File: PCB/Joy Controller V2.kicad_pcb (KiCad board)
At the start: 2 copper layers, 172.6 x 70.1 mm, 78 parts, among them J1 USB_C_Receptacle_USB2.0_16P, J2 Conn_02x16_Odd_Even, Q1 NPN, Q2 NPN, SW1 SW_Push, SW10 SW_Push, SW11 SW_Push, SW12 SW_Push, SW13 SW_Push, SW14 RotaryEncoder_Switch_MP, SW2 SW_Push, SW3 SW_Push, SW4 SW_Push, SW5 SW_Push, SW6 SW_Push, SW7 SW_Push, SW8 SW_Push, SW9 SW_Push, U1 COM-09032, U2 COM-09032, U3 MCP23017_SO, U4 ADS1015IDGS

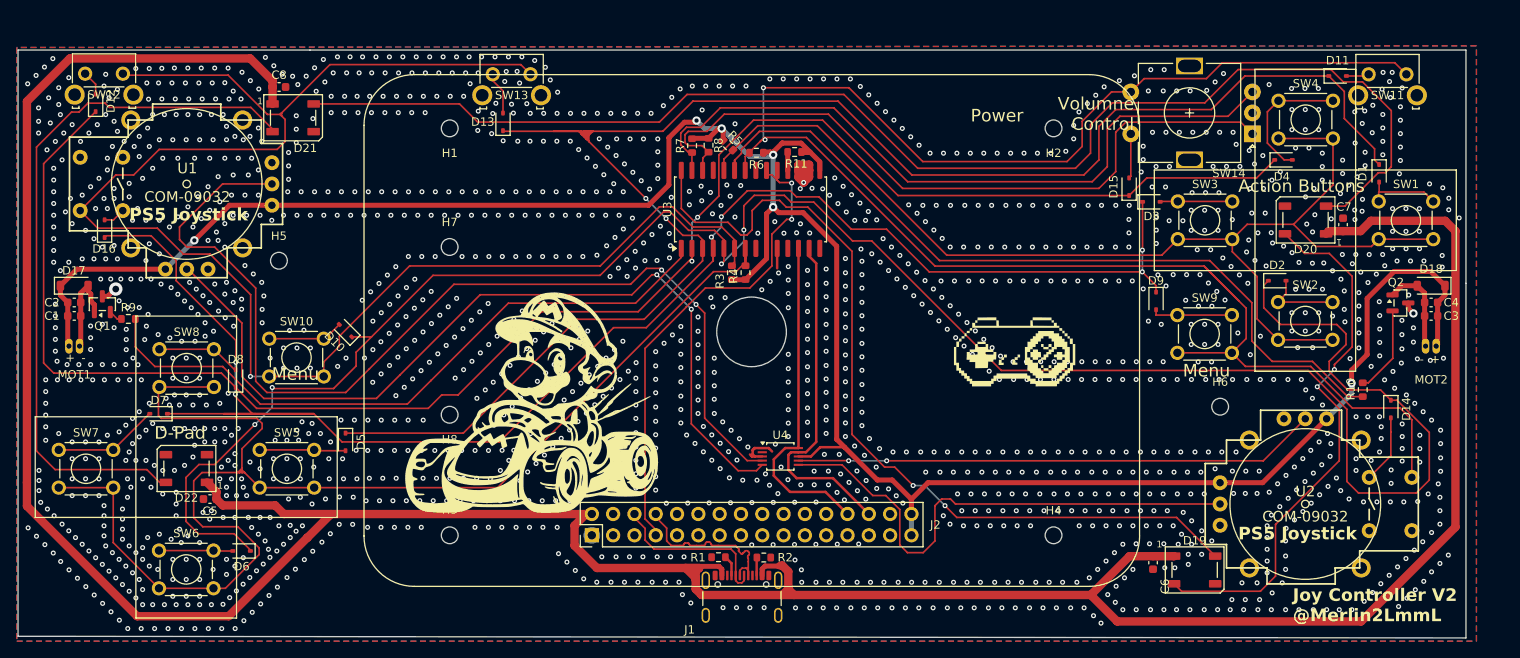
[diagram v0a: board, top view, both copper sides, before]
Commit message: Add files via upload
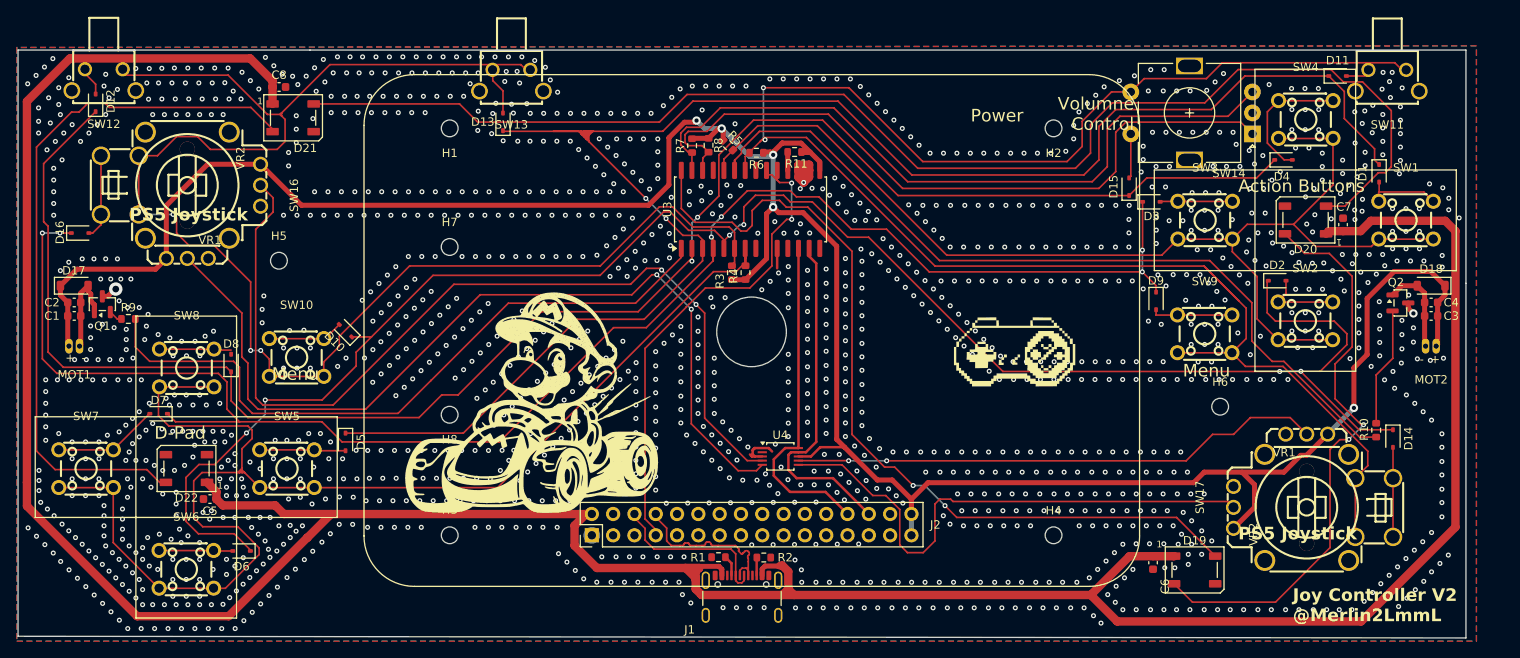
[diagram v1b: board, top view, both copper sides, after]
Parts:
- removed U1, U2: COM-09032, Joy:JOYSTICK
- added SW16: RKJXV1224005, lcsc:SW-TH_RKJXV1224005, F.Cu at (75.5, 81.0)
- added SW17: RKJXV1224005, lcsc:SW-TH_RKJXV1224005, F.Cu at (210.5, 117.0)
- SW1, SW10, SW2, SW3, SW4, SW5, SW6, SW7, SW8, SW9: value SW_Push -> B3F-1070; footprint Button_Switch_THT:SW_TH_Tactile_Omron_B3F-107x -> lcsc:SW-TH_4P-L6.2-W6.2-P4.50-LS6.5
- SW11, SW12, SW13: value SW_Push -> B3F-3152; footprint Button_Switch_THT:SW_SPST_Omron_B3F-315x_Angled -> lcsc:KEY-TH_4P-L7.3-W10.2-P4.50-LS7.0
- moved R10 5.08 mm to (218.0, 109.0)
- moved SW10 3.95 mm to (89.3, 100.3)
- moved SW3 3.95 mm to (197.6, 84.0)
- moved SW4 3.95 mm to (209.6, 72.0)
- moved SW5 3.95 mm to (88.2, 113.6)
- moved SW6 3.95 mm to (76.2, 125.6)
- moved SW7 3.95 mm to (64.2, 113.6)
- moved SW8 3.95 mm to (76.2, 101.6)
- moved SW1 3.95 mm to (221.6, 84.0)
- moved SW2 3.95 mm to (209.6, 96.0)
- moved SW9 3.95 mm to (197.6, 97.5)
- moved D14 3.53 mm to (220.0, 110.0)
- moved D16 2.97 mm to (63.5, 85.5), turned to 0 degrees
- moved SW12 2.35 mm to (66.3, 67.2), turned to 180 degrees
- moved SW13 2.35 mm to (114.9, 67.3), turned to 180 degrees
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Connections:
- D6 pad 2: Net-(D6-A) -> unconnected-(D6-A-Pad2)
- SW1 pad 2: COL1 -> Net-(D1-A)
- SW10 pad 2: COL3 -> Net-(D10-A)
- SW11 pad 2: COL0 -> Net-(D11-A)
- SW12 pad 2: COL3 -> Net-(D12-A)
- SW13 pad 2: COL3 -> Net-(D13-A)
- SW14 pad S1: COL0 -> EC11+
- SW2 pad 2: COL1 -> Net-(D2-A)
- SW3 pad 2: COL1 -> Net-(D3-A)
- SW4 pad 2: COL1 -> Net-(D4-A)
- SW5 pad 2: COL2 -> Net-(D5-A)
- SW6 pad 1: Net-(D6-A) -> unconnected-(SW6-Pad1)
- SW6 pad 2: COL2 -> unconnected-(SW6-Pad2)
- SW7 pad 2: COL2 -> Net-(D7-A)
- SW8 pad 2: COL2 -> Net-(D8-A)
- SW9 pad 2: COL0 -> Net-(D9-A)
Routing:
- net ROW1: track 252.0 -> 216.7 mm, vias 4 -> 6
- net +3.3V: track 286.0 -> 303.3 mm, vias 6 -> 5
- net JOY_L_VRx: track 121.1 -> 111.1 mm
- net Net-(D6-A): track 8.82 -> 0.00 mm
- net (no net): track 0.00 -> 8.82 mm
- net JOY_SW_L-: track 2.63 -> 10.1 mm
- net COL3: track 192.8 -> 186.1 mm, vias 1 -> 3
- net ROW2: track 203.3 -> 196.6 mm
- net Net-(D19-DOUT): track 65.0 -> 69.3 mm
- net Net-(Q2-B): track 10.5 -> 14.2 mm
- net M_HAP_R: track 94.8 -> 98.4 mm
- net JOY_L_VRy: track 102.8 -> 106.2 mm
- net JOY_SW_R-: track 8.16 -> 10.7 mm
- net M_HAP_L: track 80.3 -> 82.8 mm
- net COL2: track 162.8 -> 160.6 mm
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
